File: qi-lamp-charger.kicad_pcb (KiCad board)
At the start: 2 copper layers, 41.5 x 44 mm, 85 parts, among them J1 Conn_01x03, J2 Conn_01x02, J4 Conn_01x06, J5 Conn_01x03, Q1 BSS308PE H6327, SW1 SKTDLDE010, U1 SLG5NV1430V, U2 BQ51050BRHL, U3 ESP-12E

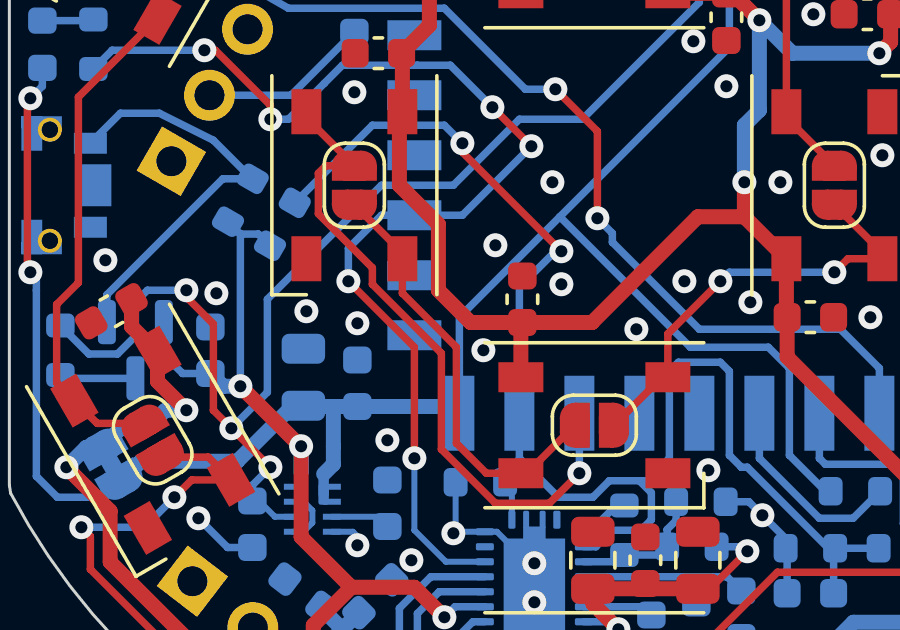
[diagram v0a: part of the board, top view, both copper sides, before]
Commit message: Shematic changed
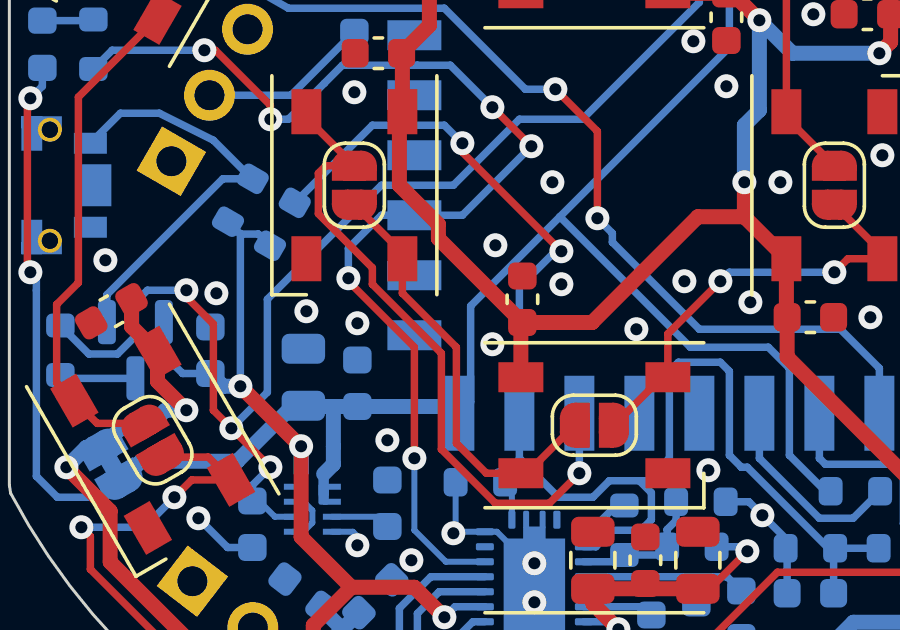
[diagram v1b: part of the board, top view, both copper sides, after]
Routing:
- net LED_V+: track 160.8 -> 159.8 mm
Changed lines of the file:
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@@
   (via (at 90.4 104.2) (size 0.8) (drill 0.4) (layers "F.Cu" "B.Cu") (net 5))
   (via (at 92.1 112) (size 0.8) (drill 0.4) (layers "F.Cu" "B.Cu") (net 5))
-  (via (at 96.3 105.5) (size 0.8) (drill 0.4) (layers "F.Cu" "B.Cu") (net 5))
+  (via (at 96.6 105.3) (size 0.8) (drill 0.4) (layers "F.Cu" "B.Cu") (net 5))
   (via (at 81.5 92.1) (size 0.8) (drill 0.4) (layers "F.Cu" "B.Cu") (net 5))
   (via (at 97.6 116.9) (size 0.8) (drill 0.4) (layers "F.Cu" "B.Cu") (net 5))
@@
   (segment (start 90.974999 110.3) (end 90.975 109.625) (width 0.35) (layer "B.Cu") (net 15))
   (segment (start 90.325 107.375) (end 90.3 107.35) (width 0.5) (layer "B.Cu") (net 15))
+  (segment (start 95.875489 107.224511) (end 95.5 107.6) (width 0.25) (layer "B.Cu") (net 15))
   (segment (start 81.4 103.1) (end 81.2 102.9) (width 0.25) (layer "B.Cu") (net 15))
   (segment (start 103.325 89.4) (end 103.125 89.6) (width 0.25) (layer "B.Cu") (net 15))
@@
   (segment (start 82.1 110.4) (end 81.4 109.7) (width 0.25) (layer "B.Cu") (net 15))
   (segment (start 88.1 109.2) (end 89.95 107.35) (width 0.5) (layer "B.Cu") (net 15))
+  (segment (start 98.85 101.05) (end 95.875489 104.024511) (width 0.25) (layer "B.Cu") (net 15))
   (segment (start 107.700978 110.2) (end 107.875 110.2) (width 0.25) (layer "B.Cu") (net 15))
   (segment (start 91.3 107.4) (end 91.325 107.375) (width 0.5) (layer "B.Cu") (net 15))
-  (segment (start 95.5 104.4) (end 95.5 105.9) (width 0.25) (layer "B.Cu") (net 15))
   (segment (start 103.2 105.4) (end 98.85 101.05) (width 0.25) (layer "B.Cu") (net 15))
   (segment (start 95.275 107.375) (end 95.5 107.6) (width 0.5) (layer "B.Cu") (net 15))
@@
   (segment (start 102.1 87) (end 102 86.9) (width 0.25) (layer "B.Cu") (net 15))
   (segment (start 104.5 89.4) (end 104.5 95.4) (width 0.25) (layer "B.Cu") (net 15))
-  (segment (start 98.85 101.05) (end 95.5 104.4) (width 0.25) (layer "B.Cu") (net 15))
+  (segment (start 95.875489 104.024511) (end 95.875489 107.224511) (width 0.25) (layer "B.Cu") (net 15))
   (segment (start 106.5 106.1) (end 105.8 105.4) (width 0.25) (layer "B.Cu") (net 15))
-  (segment (start 95.5 105.9) (end 95.5 107.6) (width 0.25) (layer "B.Cu") (net 15))
   (segment (start 112.870636 90.937083) (end 114.397432 90.937083) (width 0.25) (layer "F.Cu") (net 16))
   (segment (start 112.1 85.2) (end 112.1 90.166447) (width 0.25) (layer "F.Cu") (net 16))
@@
   (segment (start 106.4 104.375) (end 106.425 104.4) (width 0.5) (layer "F.Cu") (net 23))
   (segment (start 104.4 93.625) (end 104.625 93.625) (width 0.5) (layer "F.Cu") (net 23))
-  (segment (start 93.5 100) (end 94.8 101.3) (width 0.5) (layer "F.Cu") (net 23))
   (segment (start 112.111791 109.821762) (end 111.933553 110) (width 0.5) (layer "F.Cu") (net 23))
+  (segment (start 94.8 101.775) (end 97.6 104.575) (width 0.5) (layer "F.Cu") (net 23))
   (segment (start 110.698609 110) (end 106.425 105.726391) (width 0.5) (layer "F.Cu") (net 23))
   (segment (start 86.4 107.5) (end 85.438209 106.538209) (width 0.5) (layer "F.Cu") (net 23))
   (segment (start 106.4 104.375) (end 106.375 104.4) (width 0.5) (layer "F.Cu") (net 23))
   (segment (start 85.438209 106.538209) (end 85.438209 105.578238) (width 0.5) (layer "F.Cu") (net 23))
-  (segment (start 94.8 101.3) (end 94.8 103.5) (width 0.5) (layer "F.Cu") (net 23))
   (segment (start 99.925 104.575) (end 103.449999 101.050001) (width 0.5) (layer "F.Cu") (net 23))
-  (segment (start 93.6 97.55) (end 93.5 97.65) (width 0.5) (layer "F.Cu") (net 23))
   (segment (start 95.625 115.4) (end 95.5 115.525) (width 0.5) (layer "F.Cu") (net 23))
   (segment (start 83.859394 110.859394) (end 82.4 109.4) (width 0.5) (layer "F.Cu") (net 23))
@@
   (segment (start 87.888209 90.178238) (end 87.888209 89.270461) (width 0.5) (layer "F.Cu") (net 23))
   (segment (start 105 101.050001) (end 106.4 102.450001) (width 0.5) (layer "F.Cu") (net 23))
-  (segment (start 94.8 103.5) (end 95.875 104.575) (width 0.5) (layer "F.Cu") (net 23))
+  (segment (start 93.6 97.55) (end 93.5 97.65) (width 0.5) (layer "F.Cu") (net 23))
   (segment (start 97.55 104.625) (end 97.6 104.575) (width 0.5) (layer "F.Cu") (net 23))
   (segment (start 92.9 86.7) (end 94.5 88.3) (width 0.5) (layer "F.Cu") (net 23))
@@
   (segment (start 93.575 115.525) (end 95.5 115.525) (width 0.5) (layer "F.Cu") (net 23))
   (segment (start 91.6 86.7) (end 92.9 86.7) (width 0.5) (layer "F.Cu") (net 23))
+  (segment (start 93.5 100) (end 94.8 101.3) (width 0.5) (layer "F.Cu") (net 23))
   (segment (start 91.3 117.8) (end 93.575 115.525) (width 0.5) (layer "F.Cu") (net 23))
   (segment (start 88.55 116.4) (end 89.95 117.8) (width 0.5) (layer "F.Cu") (net 23))
+  (segment (start 93.5 97.65) (end 93.5 100) (width 0.5) (layer "F.Cu") (net 23))
   (segment (start 87.3 116) (end 83.859394 112.559394) (width 0.5) (layer "F.Cu") (net 23))
   (segment (start 90.0125 88.2875) (end 91.6 86.7) (width 0.5) (layer "F.Cu") (net 23))
@@
   (segment (start 95.475 115.525) (end 95.5 115.525) (width 0.5) (layer "F.Cu") (net 23))
   (segment (start 88.87117 88.2875) (end 90.0125 88.2875) (width 0.5) (layer "F.Cu") (net 23))
+  (segment (start 94.8 101.3) (end 94.8 101.775) (width 0.5) (layer "F.Cu") (net 23))
   (segment (start 102.45 84.6) (end 104.375 84.6) (width 0.5) (layer "F.Cu") (net 23))
   (segment (start 109.875 89.734971) (end 109.875 89.425) (width 0.25) (layer "F.Cu") (net 23))
   (segment (start 103.449999 101.050001) (end 105 101.050001) (width 0.5) (layer "F.Cu") (net 23))
-  (segment (start 93.5 97.65) (end 93.5 100) (width 0.5) (layer "F.Cu") (net 23))
-  (segment (start 95.875 104.575) (end 97.6 104.575) (width 0.5) (layer "F.Cu") (net 23))
   (segment (start 106.425 105.726391) (end 106.425 104.4) (width 0.5) (layer "F.Cu") (net 23))
   (segment (start 104.375 84.6) (end 104.4 84.625) (width 0.5) (layer "F.Cu") (net 23))
@@
   (segment (start 103.5 104.8) (end 108.2 104.8) (width 0.25) (layer "B.Cu") (net 48))
   (segment (start 89.2 97.334643) (end 89.2 97.8) (width 0.25) (layer "F.Cu") (net 49))
+  (segment (start 91.8 103.1) (end 91.8 103.2) (width 0.25) (layer "F.Cu") (net 49))
+  (segment (start 87 95.5) (end 87.365357 95.5) (width 0.25) (layer "F.Cu") (net 49))
   (segment (start 94 105.4) (end 94 109.1) (width 0.25) (layer "F.Cu") (net 49))
-  (segment (start 87 95.5) (end 87.365357 95.5) (width 0.25) (layer "F.Cu") (net 49))
   (segment (start 91.8 103.2) (end 94 105.4) (width 0.25) (layer "F.Cu") (net 49))
   (segment (start 87.365357 95.5) (end 89.2 97.334643) (width 0.25) (layer "F.Cu") (net 49))
@@
   (via (at 89.2 97.8) (size 0.8) (drill 0.4) (layers "F.Cu" "B.Cu") (net 49))
   (via (at 94 109.1) (size 0.8) (drill 0.4) (layers "F.Cu" "B.Cu") (net 49))
-  (via (at 91.8 103.2) (size 0.8) (drill 0.4) (layers "F.Cu" "B.Cu") (net 49))
+  (via (at 91.8 103.1) (size 0.8) (drill 0.4) (layers "F.Cu" "B.Cu") (net 49))
   (via (at 87 95.5) (size 0.8) (drill 0.4) (layers "F.Cu" "B.Cu") (net 49))
+  (segment (start 91.8 102.1) (end 92.9 101) (width 0.25) (layer "B.Cu") (net 49))
   (segment (start 95.2 96) (end 94.1 96) (width 0.25) (layer "B.Cu") (net 49))
   (segment (start 91.6 96) (end 91 96.6) (width 0.25) (layer "B.Cu") (net 49))
@@
   (segment (start 94 109.1) (end 94 111.5) (width 0.2) (layer "B.Cu") (net 49))
   (segment (start 94.1 96) (end 91.6 96) (width 0.25) (layer "B.Cu") (net 49))
+  (segment (start 92.9 101) (end 94 101) (width 0.25) (layer "B.Cu") (net 49))
   (segment (start 83.925001 95.5) (end 83.300002 96.124999) (width 0.25) (layer "B.Cu") (net 49))
   (segment (start 87 95.5) (end 83.925001 95.5) (width 0.25) (layer "B.Cu") (net 49))
@@
   (segment (start 96.6 97.4) (end 95.2 96) (width 0.25) (layer "B.Cu") (net 49))
   (segment (start 89.8 97.8) (end 89.2 97.8) (width 0.25) (layer "B.Cu") (net 49))
-  (segment (start 91.8 102.1) (end 92.9 101) (width 0.25) (layer "B.Cu") (net 49))
-  (segment (start 92.9 101) (end 94 101) (width 0.25) (layer "B.Cu") (net 49))
   (segment (start 91 96.6) (end 89.8 97.8) (width 0.25) (layer "B.Cu") (net 49))
   (segment (start 95.6 101) (end 97.9 98.7) (width 0.25) (layer "B.Cu") (net 49))
   (segment (start 95.05 112.55) (end 96.349998 112.55) (width 0.2) (layer "B.Cu") (net 49))
-  (segment (start 91.8 103.2) (end 91.8 102.1) (width 0.25) (layer "B.Cu") (net 49))
+  (segment (start 91.8 103.1) (end 91.8 102.1) (width 0.25) (layer "B.Cu") (net 49))
   (segment (start 95.6 98.6) (end 95.6 98.9) (width 0.25) (layer "F.Cu") (net 51))
   (segment (start 95.6 98.9) (end 98.9 102.2) (width 0.25) (layer "F.Cu") (net 51))
